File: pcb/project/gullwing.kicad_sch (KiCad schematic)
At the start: 7 parts

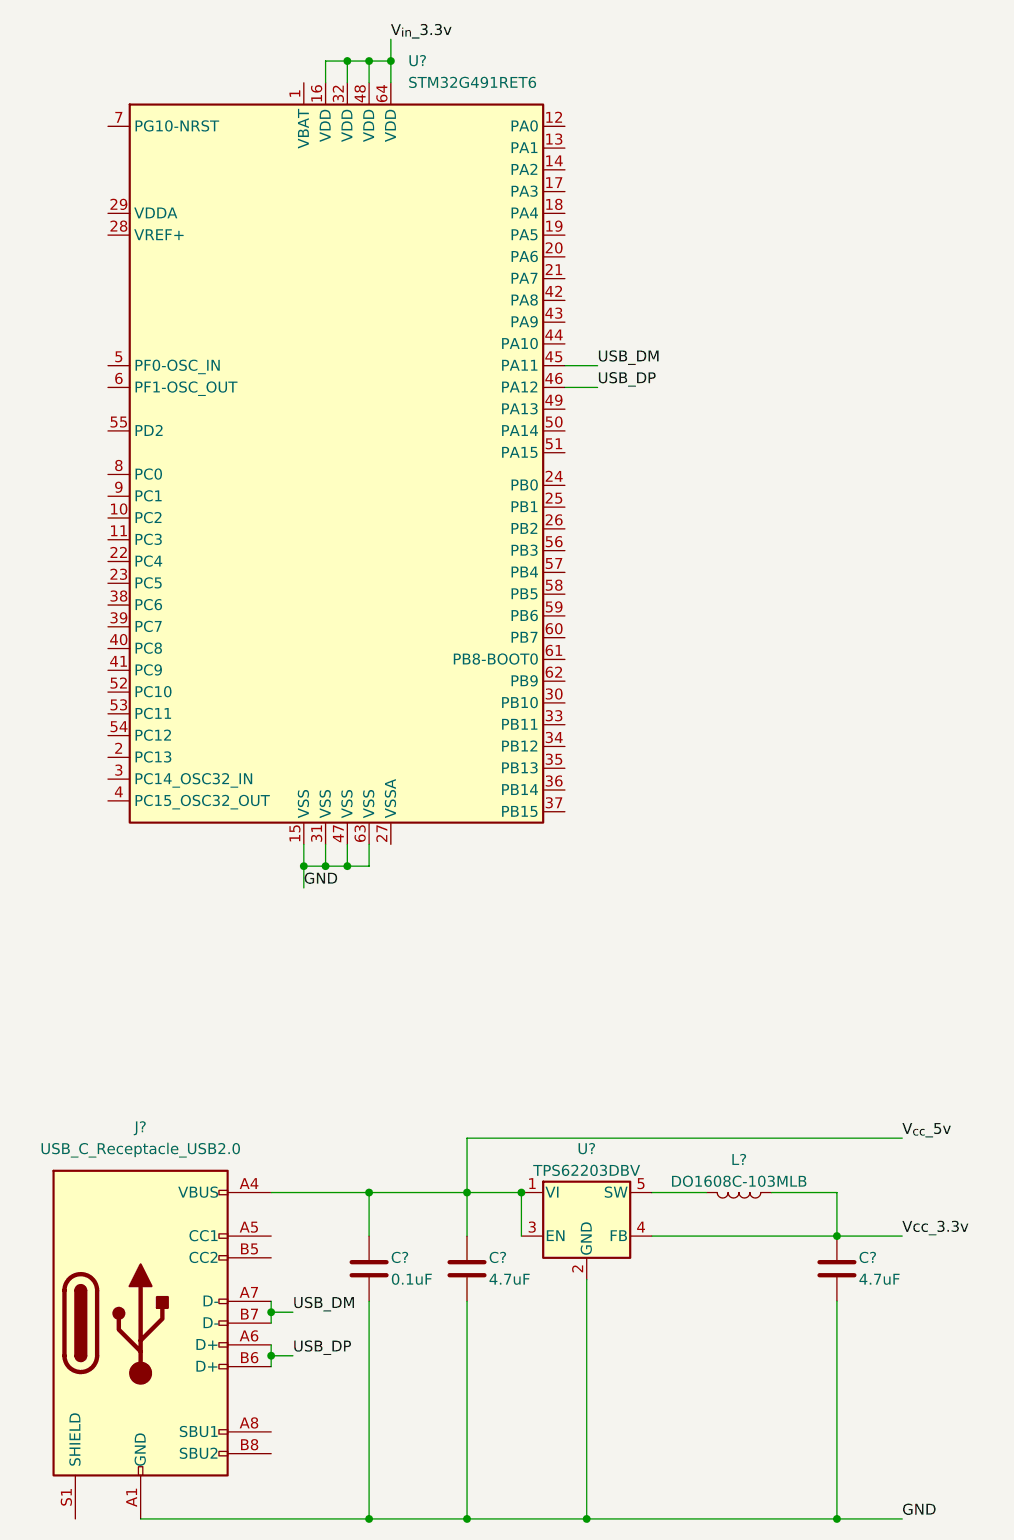
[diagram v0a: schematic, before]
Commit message: wip
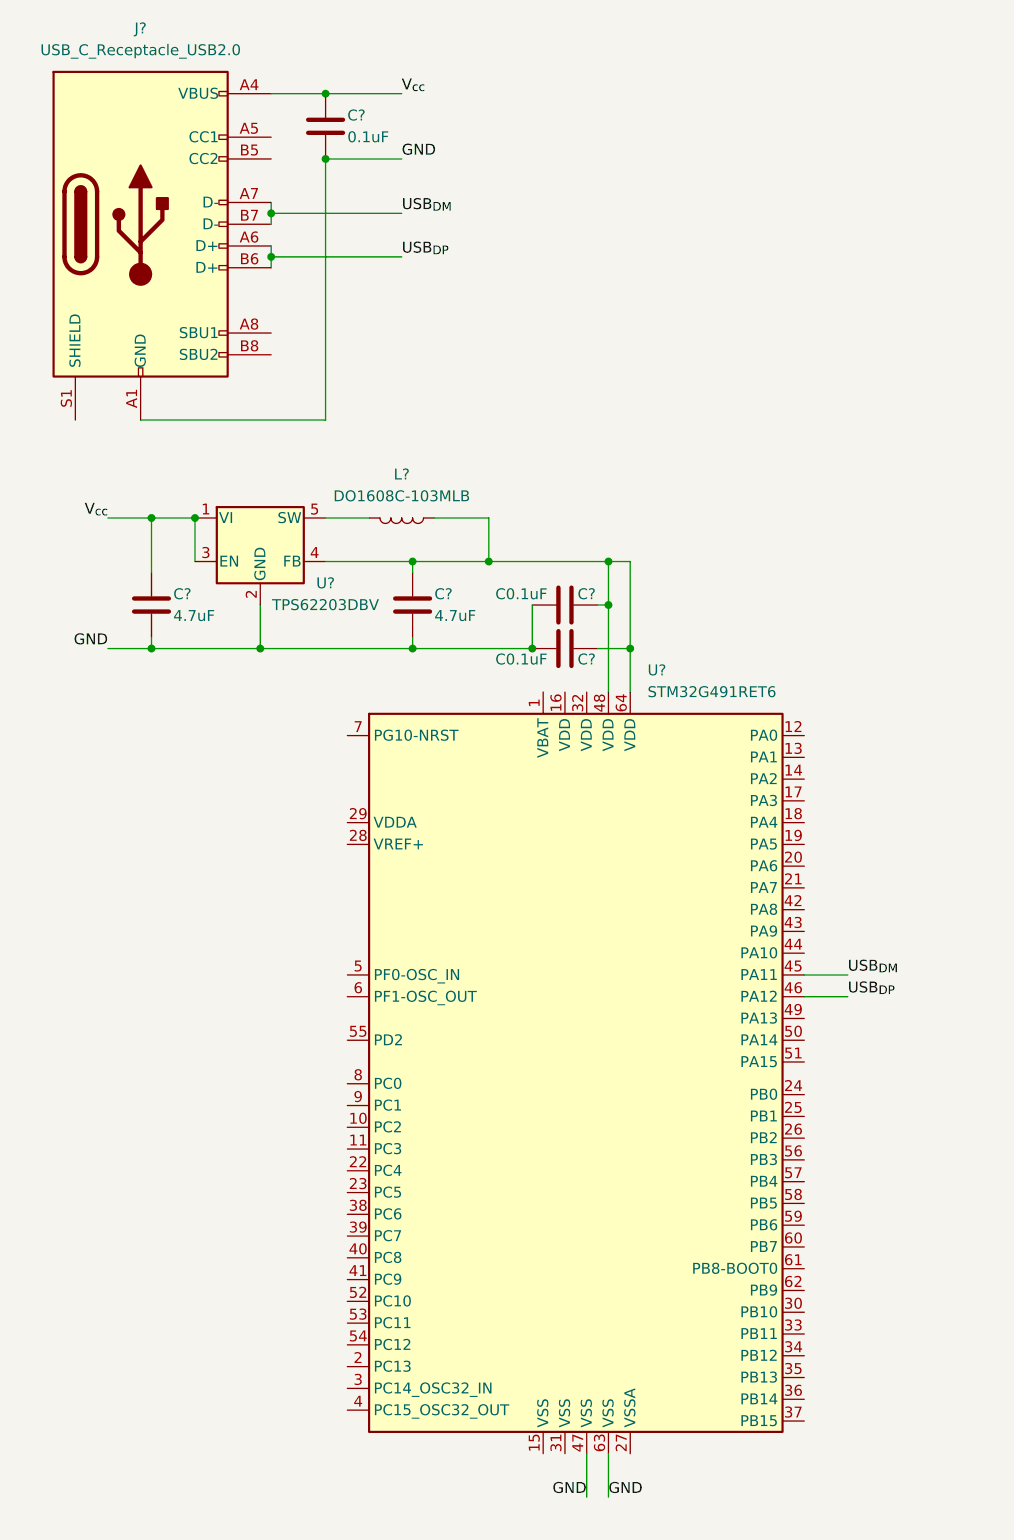
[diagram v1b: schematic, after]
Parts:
- removed C? (x2): 4.7uF, symbol Device:C
- removed C?: 0.1uF, symbol Device:C
- removed L?: DO1608C-103MLB, Inductors:DO1608C, symbol Device:L
- removed U?: TPS62203DBV, Package_TO_SOT_SMD:SOT-23-5, symbol Regulator_Switching:TPS62203DBV
- added C? (x2): C0.1uF, symbol Device:C
- added C? (x2): 4.7uF, symbol Device:C
- added C?: 0.1uF, symbol Device:C
- added L?: DO1608C-103MLB, Inductors:DO1608C, symbol Device:L
- added U?: TPS62203DBV, Package_TO_SOT_SMD:SOT-23-5, symbol Regulator_Switching:TPS62203DBV
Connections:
- net GND: now also C?.1, C?.2, C?.2, C?.2, C?.2, U?.2 (GND); no longer U?.15 (VSS), U?.31 (VSS)
- net USB_DM renamed USB_{DM}
- net USB_DP renamed USB_{DP}
- net V_{cc}_5v renamed V_{cc}
- net V_{cc}: now also C?.1, C?.1, U?.1 (VI), U?.3 (EN)
- net V_{in}_3.3v: no longer names the net of U?.48 (VDD), U?.64 (VDD)
- net V_{in}_3.3v: now also C?.1, C?.1, C?.2, L?.1, U?.4 (FB); no longer U?.16 (VDD), U?.32 (VDD)
- new net: L?.2, U?.5 (SW)
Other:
- moved on the sheet: J?, U?
